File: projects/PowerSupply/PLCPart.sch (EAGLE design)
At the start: 44 parts, among them IC1 L7818CV, IC2 L7918CV, IC3 LM2574N-5.0, IC4 LM2574N-5.0, IC5 L7915CV, IC6 L7815CV, IC7 LM358N, IC8 LM358N, X1 MCU-PWR, X2 MCU-IN, X4 MCU-OUT

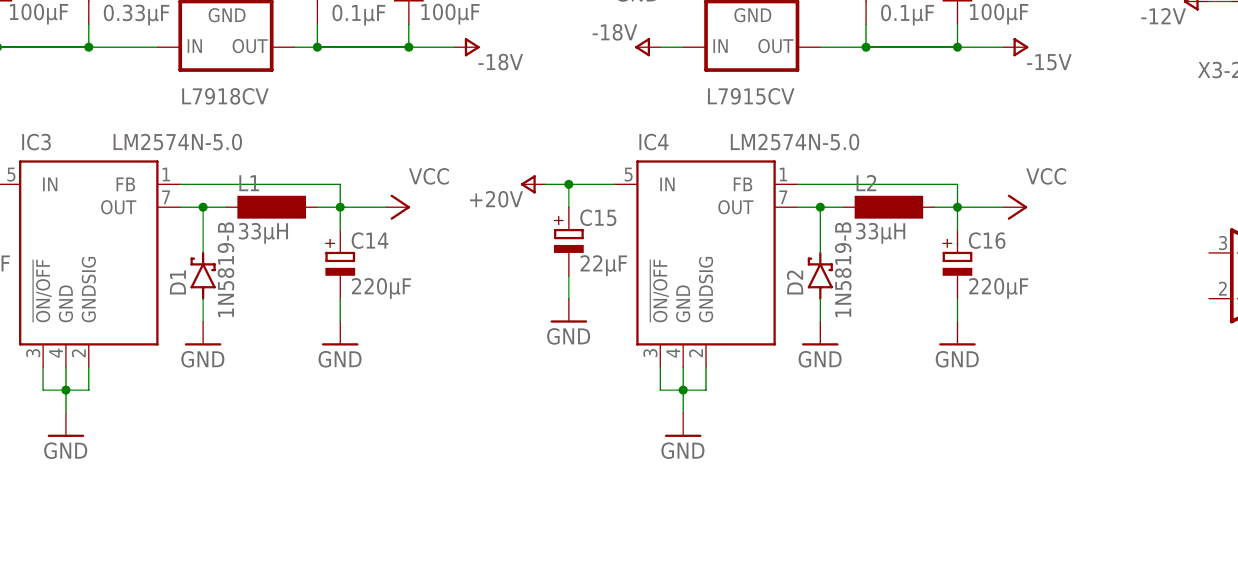
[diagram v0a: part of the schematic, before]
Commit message: feat: plc part modified
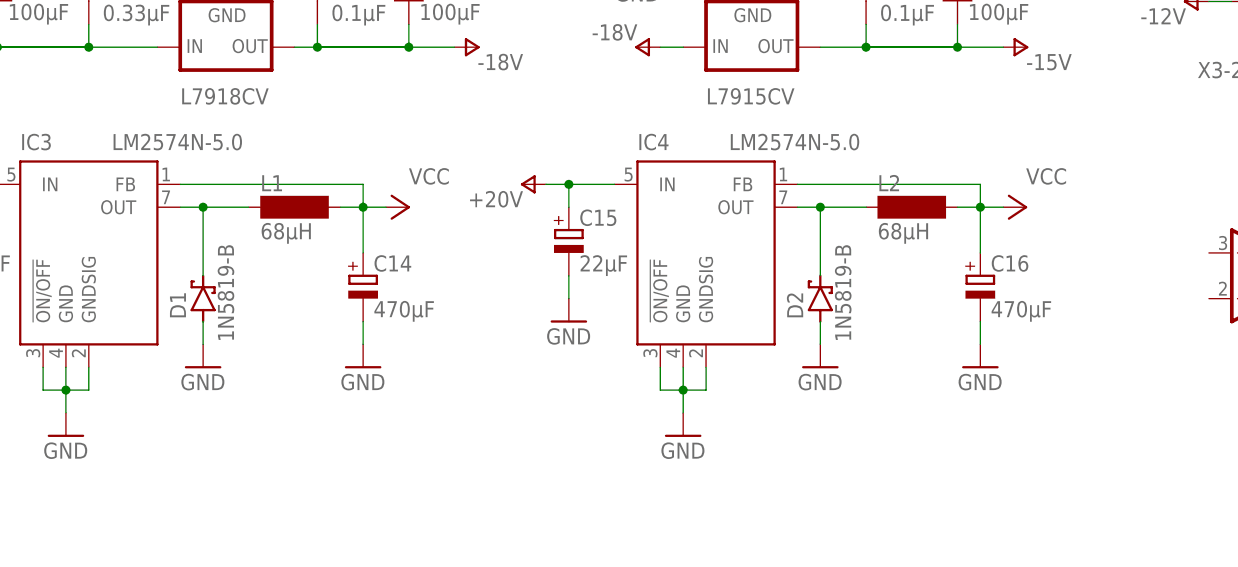
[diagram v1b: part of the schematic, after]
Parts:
- C14, C16: value 220µF -> 470µF
- L1, L2: value 33µH -> 68µH; device inductor-neosid:SD12-680 -> inductor-neosid:SD12K100
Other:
- moved on the sheet: C14, C16, D1, D2, L1, L2
